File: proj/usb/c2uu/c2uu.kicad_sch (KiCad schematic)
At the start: 1 part, among them J1 USB_C_Receptacle_USB2.0_16P

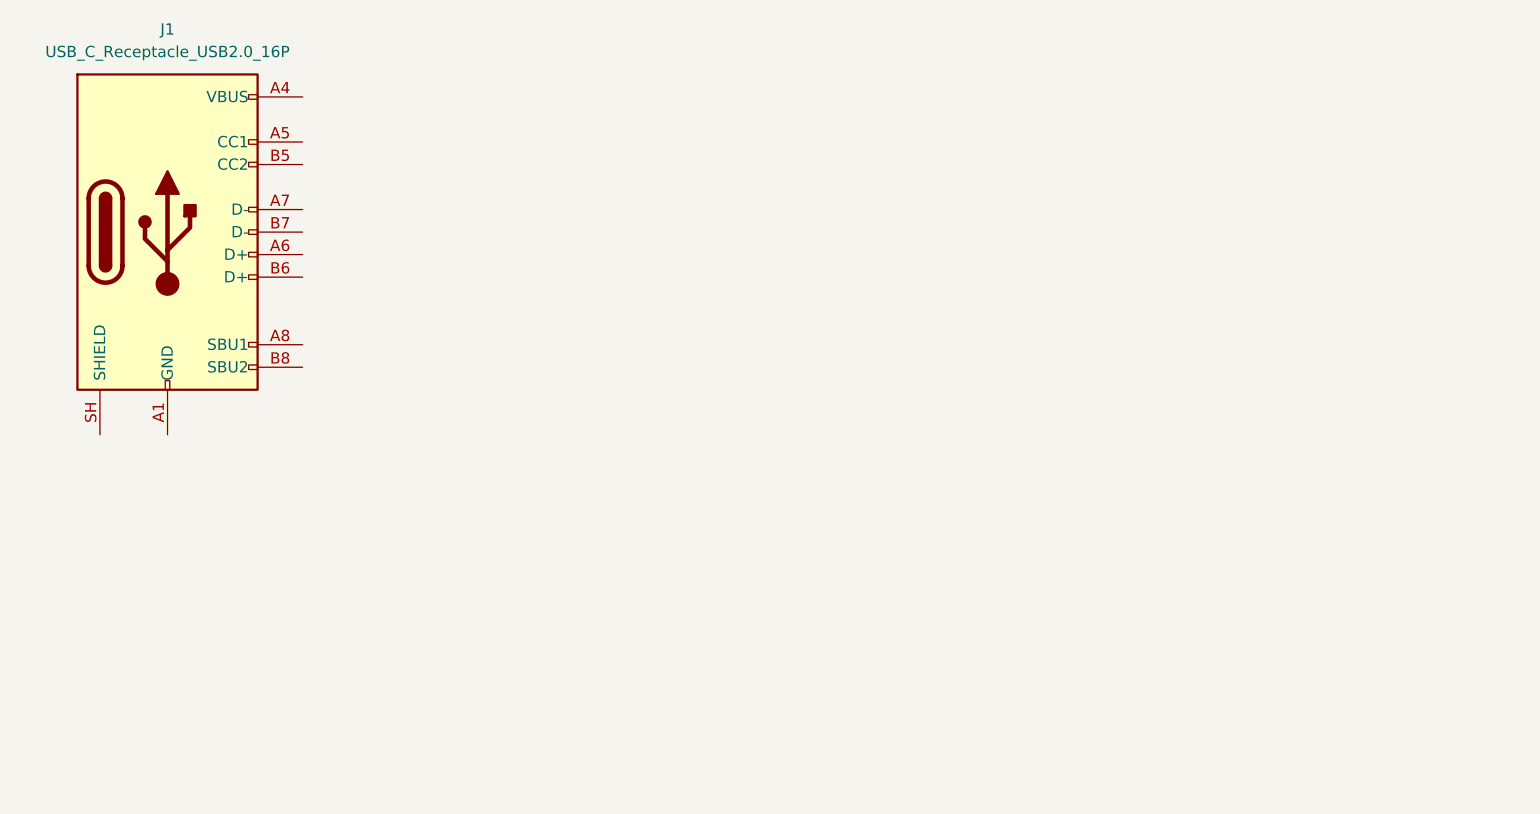
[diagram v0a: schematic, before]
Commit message: -
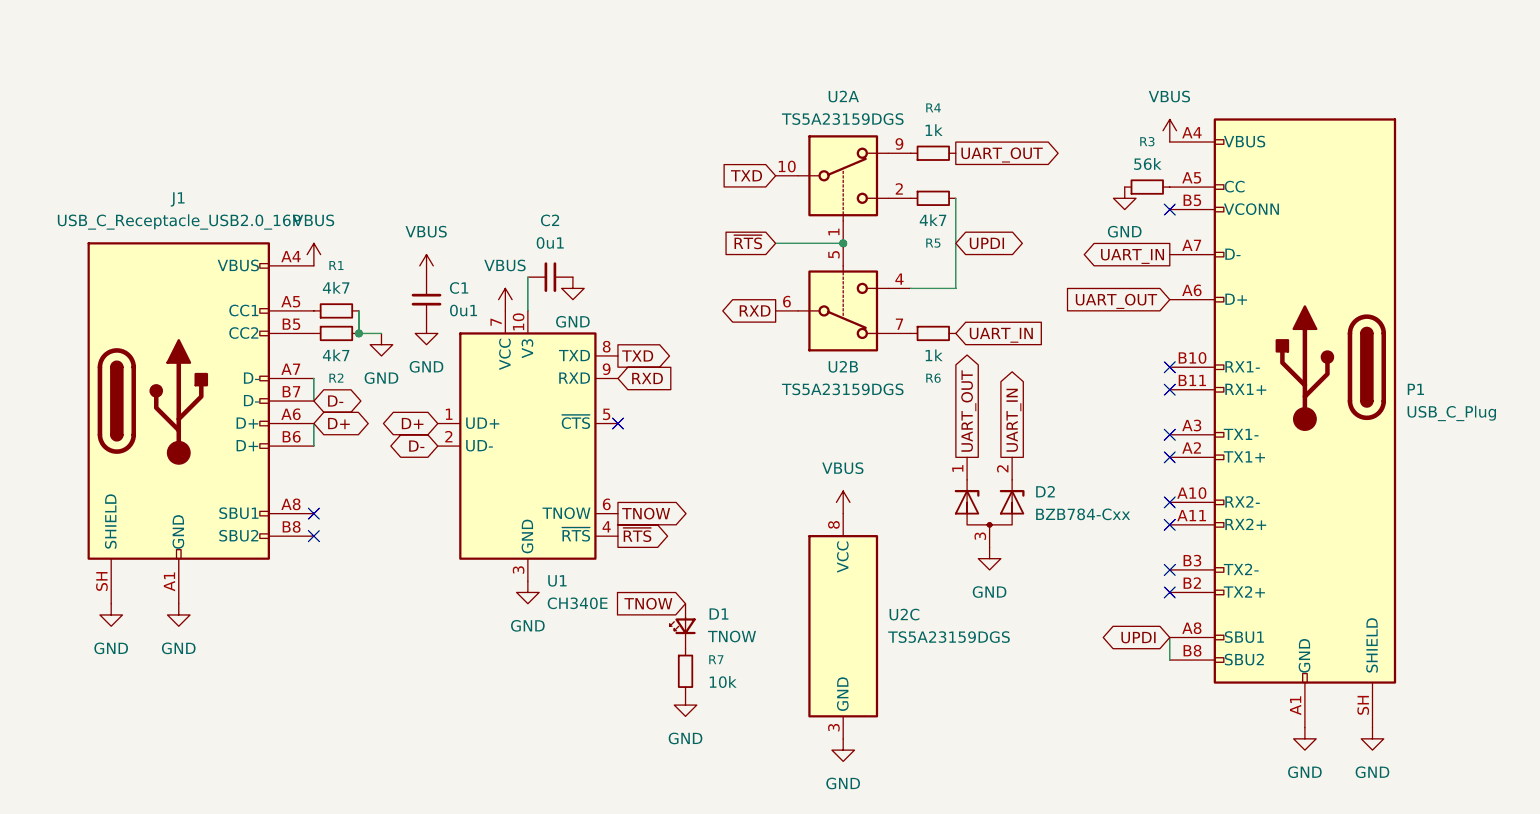
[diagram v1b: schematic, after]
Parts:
- added C1, C2: 0u1, Capacitor_SMD:C_0603_1608Metric, symbol Device:C_Small
- added D1: TNOW, LED_SMD:LED_0603_1608Metric, symbol Device:LED_Small
- added D2: BZB784-Cxx, Package_TO_SOT_SMD:SOT-323_SC-70, symbol Library:BZB784-Cxx
- added P1: USB_C_Plug, Connector_USB:USB_C_Plug_Molex_105444, symbol Connector:USB_C_Plug
- added R1, R2, R5: 4k7, Resistor_SMD:R_0603_1608Metric, symbol Device:R_Small
- added R3: 56k, Resistor_SMD:R_0603_1608Metric, symbol Device:R_Small
- added R4, R6: 1k, Resistor_SMD:R_0603_1608Metric, symbol Device:R_Small
- added R7: 10k, Resistor_SMD:R_0603_1608Metric, symbol Device:R_Small
- added U1: CH340E, Package_SO:MSOP-10_3x3mm_P0.5mm, symbol Interface_USB:CH340E
- added U2: TS5A23159DGS, Package_SO:TSSOP-10_3x3mm_P0.5mm, symbol Analog_Switch:TS5A23159DGS
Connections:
- net GND: now reaches J1.A1 (GND), J1.A12 (GND), J1.B1 (GND), J1.B12 (GND)
- net GND: now also J1.SH (SHIELD), C1.2, C2.2, D2.3 (A), P1.A1 (GND), P1.A12 (GND), P1.B1 (GND), P1.B12 (GND), P1.SH (SHIELD), R1.2, R2.2, R3.1, R7.2, U1.3 (GND), U2.3 (GND)
- net VBUS: now reaches J1.A4 (VBUS), J1.A9 (VBUS), J1.B4 (VBUS), J1.B9 (VBUS)
- net VBUS: now also C1.1, P1.A4 (VBUS), P1.A9 (VBUS), P1.B4 (VBUS), P1.B9 (VBUS), U1.7 (VCC), U2.8 (VCC)
- net at J1.A5 (CC1): now also R1.1
- net D+: now reaches J1.A6 (D+)
- net D+: now also J1.B6 (D+), U1.1 (UD+)
- net D-: now reaches J1.A7 (D-)
- net D-: now also J1.B7 (D-), U1.2 (UD-)
- net at J1.B5 (CC2): now also R2.1
- new net: D1.1 (K), R7.1
- new net: C2.1, U1.10 (V3)
- new net: R5.1, U2.2
- new net: R4.1, U2.9
- new net: P1.A5 (CC), R3.2
- new net: R6.1, U2.7
- new net RXD: U1.9 (RXD), U2.6
- new net TNOW: D1.2 (A), U1.6 (TNOW)
- new net TXD: U1.8 (TXD), U2.10
- new net UART_IN: D2.2 (K), P1.A7 (D-), R6.2
- new net UART_OUT: D2.1 (K), P1.A6 (D+), R4.2
- new net UPDI: P1.A8 (SBU1), P1.B8 (SBU2), R5.2, U2.4
- new net ~{RTS}: U1.4 (~{RTS}), U2.1, U2.5
- no-connect marks 0 -> 12
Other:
- moved on the sheet: J1

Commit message: -
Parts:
- P1: footprint Connector_USB:USB_C_Plug_Molex_105444 -> Library:USB_C_Plug_24P
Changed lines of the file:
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@@
 			)
 		)
-		(property "Footprint" "Connector_USB:USB_C_Plug_Molex_105444"
+		(property "Footprint" "Library:USB_C_Plug_24P"
 			(at 170.18 60.96 0)
 			(hide yes)
